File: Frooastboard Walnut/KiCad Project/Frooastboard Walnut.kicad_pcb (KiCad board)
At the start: 2 copper layers, 357.2 x 100 mm, 172 parts, among them SW1 SW_Push, U1 ATmega32U4-A, Y1 Crystal_GND24_Small

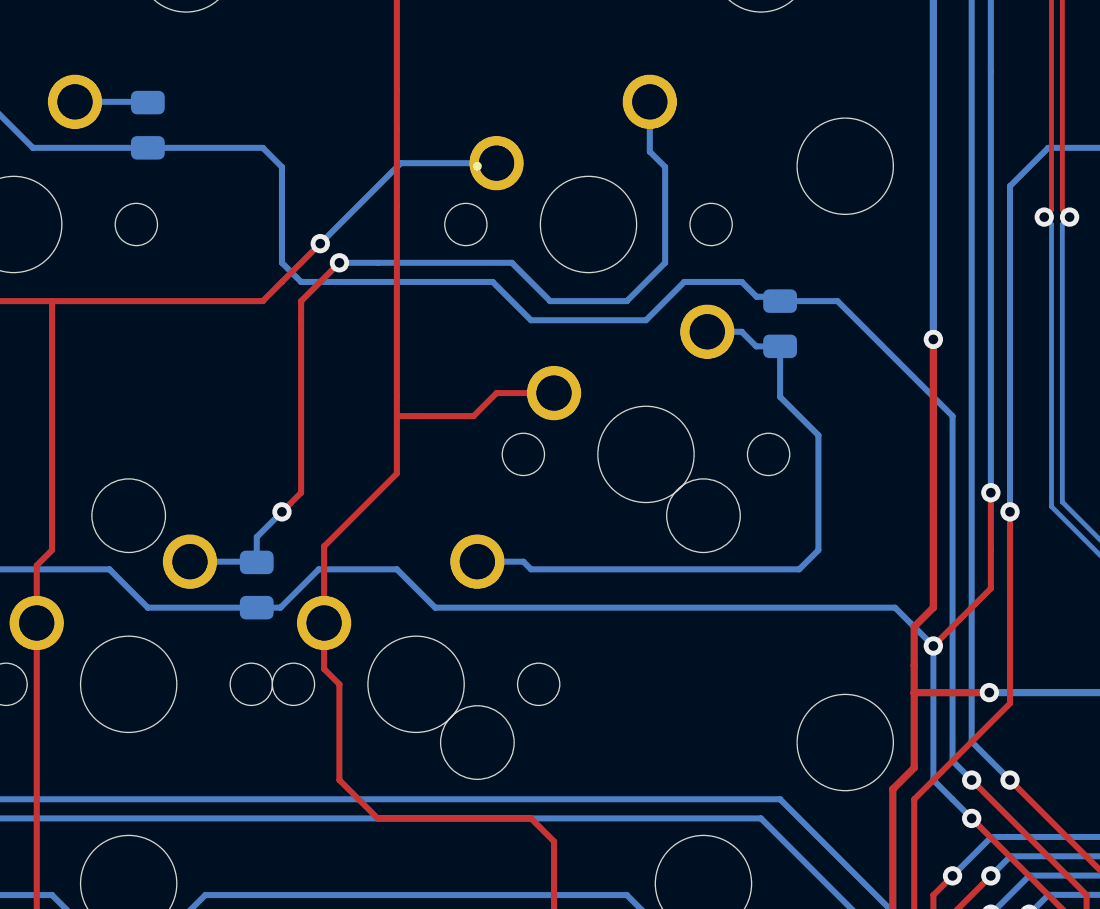
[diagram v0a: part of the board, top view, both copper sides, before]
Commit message: rotate iso enter switch
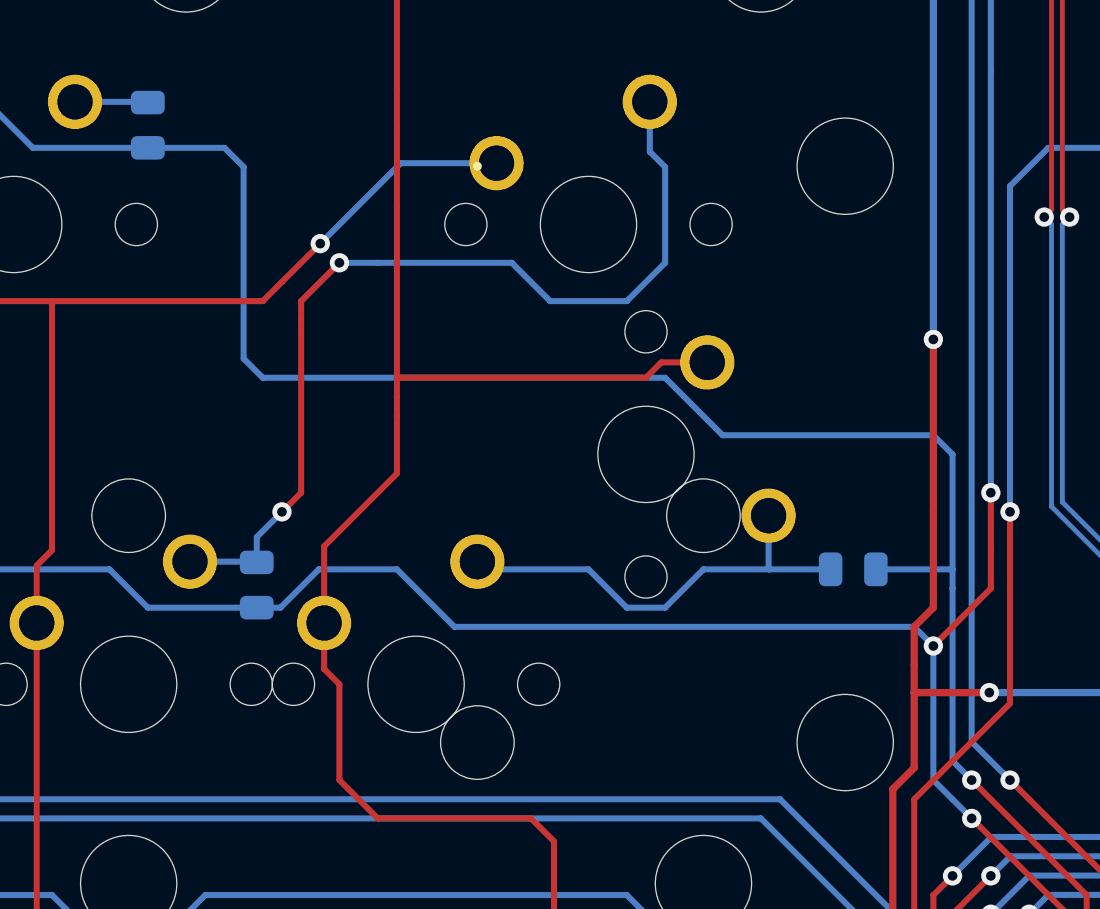
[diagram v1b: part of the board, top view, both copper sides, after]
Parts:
- KEY_ENTER1: footprint MX_Only:MXOnly-ISO-NoLED-NoStabilizers -> MX_Only:MXOnly-ISO-ROTATED-NoLED-NoStabilizers
- moved D52 10.6 mm to (303.9, 64.3), turned to 180 degrees
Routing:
- net Net-(D52-Pad2): track 27.0 -> 18.3 mm
- net COL5: track 428.3 -> 434.5 mm
- net ROW3: track 216.7 -> 219.9 mm
